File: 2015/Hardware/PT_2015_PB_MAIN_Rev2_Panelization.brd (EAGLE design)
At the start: 142.5 x 234.8 mm, 161 parts, among them Q1 Q_ACS711LC_SKETCH, Q11 Q_IRFS7437PbF, Q12 2N7002, Q14 Q_IRFS7437PbF, Q16 Q_IRFS7437PbF, Q18 Q_FDT86102LZ, Q20 Q_IRFS7437PbF, Q4 Q_ACS711LC, Q5 Q_ACS711LC, Q6 Q_IRFS7437PbF, Q7 Q_IRFS7437PbF, Q9 Q_IRFS7437PbF

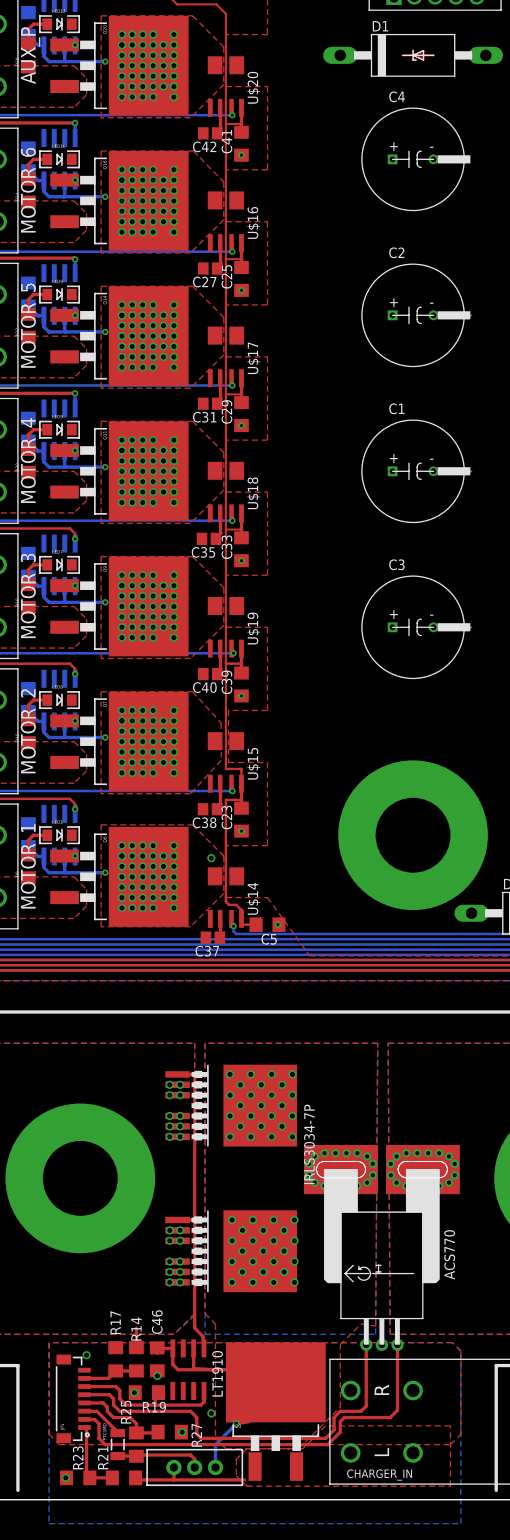
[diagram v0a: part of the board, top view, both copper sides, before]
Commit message: Cleaned up my idiotic TSTOP
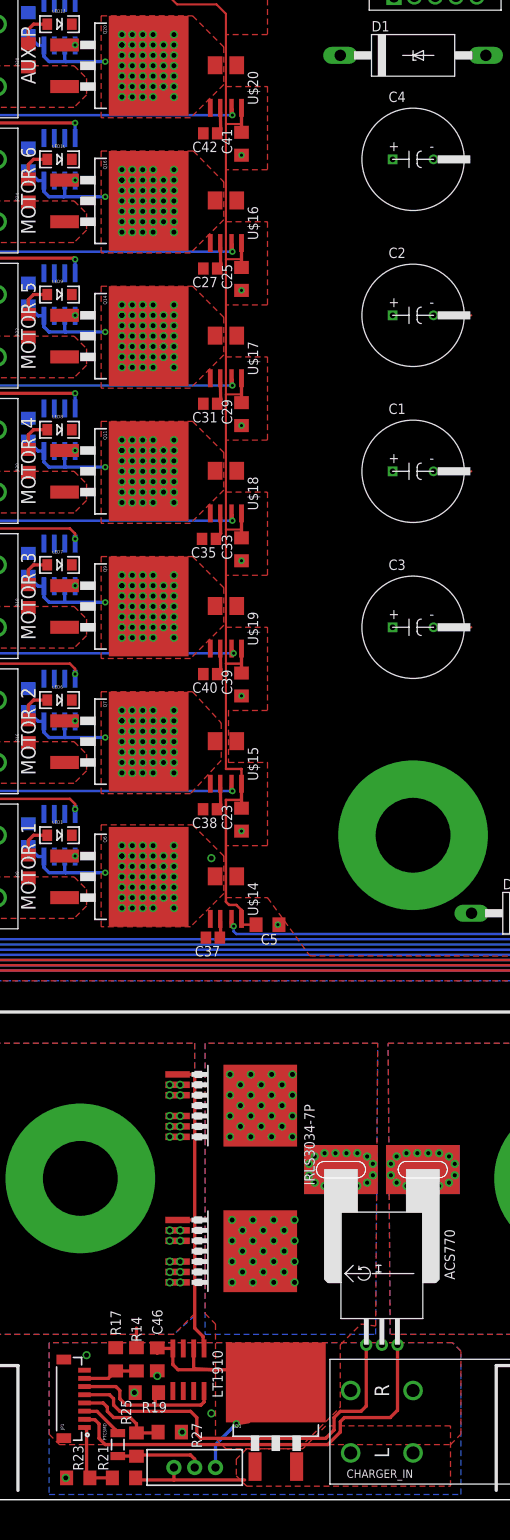
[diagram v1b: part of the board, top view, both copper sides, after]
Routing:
- net N$33: track 10.2 -> 0.00 mm
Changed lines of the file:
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@@
 <vertex x="5.08" y="2.54"/>
 </polygon>
-<dimension x1="137.795" y1="166.37" x2="137.795" y2="-67.945" x3="180.34" y3="49.2125" textsize="1.778" layer="21" unit="inch"/>
 <wire x1="1.27" y1="-8.89" x2="104.14" y2="-8.89" width="0.4064" layer="21"/>
 <wire x1="1.27" y1="-8.89" x2="1.27" y2="-52.07" width="0.4064" layer="21"/>
@@
 <wire x1="73.66" y1="-52.07" x2="104.14" y2="-52.07" width="0.4064" layer="21"/>
 <wire x1="104.14" y1="-52.07" x2="104.14" y2="-8.89" width="0.4064" layer="21"/>
+<dimension x1="137.795" y1="166.37" x2="137.541" y2="-68.453" x3="165.69279375" y3="48.928184375" textsize="3.81" layer="29" unit="inch" visible="yes"/>
 <polygon width="0.8128" layer="29">
-<vertex x="45.466" y="119.888"/>
-<vertex x="45.466" y="110.998"/>
-<vertex x="40.894" y="110.998"/>
-<vertex x="40.894" y="103.886"/>
-<vertex x="45.466" y="103.886"/>
-<vertex x="57.658" y="103.886"/>
-<vertex x="57.658" y="105.918"/>
-<vertex x="51.562" y="105.918"/>
-<vertex x="51.562" y="109.728"/>
-<vertex x="51.562" y="111.506"/>
-<vertex x="62.992" y="111.506"/>
-<vertex x="75.184" y="111.506"/>
-<vertex x="75.184" y="105.918"/>
-<vertex x="69.342" y="105.918"/>
-<vertex x="69.342" y="104.14"/>
-<vertex x="82.042" y="104.14"/>
-<vertex x="82.042" y="120.396"/>
-<vertex x="45.466" y="120.396"/>
+<vertex x="71.882" y="1.27"/>
+<vertex x="71.882" y="1.27"/>
+<vertex x="72.136" y="1.27"/>
 </polygon>
 <polygon width="0.8128" layer="29">
-<vertex x="57.658" y="104.902"/>
-<vertex x="69.342" y="104.902"/>
-<vertex x="69.342" y="104.14"/>
-<vertex x="57.658" y="104.14"/>
-<vertex x="57.658" y="103.886"/>
-</polygon>
-<polygon width="0.8128" layer="29">
-<vertex x="63.754" y="104.394"/>
-<vertex x="63.754" y="101.854"/>
-<vertex x="64.516" y="101.854" curve="-90"/>
-<vertex x="71.12" y="95.25" curve="-96.025575"/>
-<vertex x="63.5" y="88.392"/>
-<vertex x="63.5" y="83.058"/>
-<vertex x="64.516" y="83.058" curve="-90"/>
-<vertex x="71.374" y="76.2" curve="-97.62815"/>
-<vertex x="63.246" y="69.088"/>
-<vertex x="63.5" y="69.088"/>
-<vertex x="63.5" y="64.008"/>
-<vertex x="64.516" y="64.008" curve="-90"/>
-<vertex x="71.374" y="57.15" curve="-95.631113"/>
-<vertex x="63.246" y="49.784"/>
-<vertex x="63.246" y="44.958"/>
-<vertex x="64.77" y="44.958" curve="-90"/>
-<vertex x="71.628" y="38.1" curve="-90"/>
-<vertex x="64.516" y="30.988"/>
-<vertex x="63.246" y="30.988"/>
-<vertex x="63.246" y="6.35"/>
-<vertex x="81.026" y="6.35"/>
-<vertex x="81.026" y="23.622"/>
-<vertex x="79.248" y="23.622"/>
-<vertex x="79.248" y="26.67"/>
-<vertex x="81.026" y="26.67"/>
-<vertex x="81.026" y="53.594"/>
-<vertex x="80.01" y="53.594"/>
-<vertex x="80.01" y="104.14"/>
-<vertex x="73.914" y="104.14"/>
-<vertex x="73.914" y="104.394"/>
-</polygon>
-<polygon width="0.8128" layer="29">
-<vertex x="62.992" y="104.648"/>
-<vertex x="62.992" y="102.108"/>
-<vertex x="62.738" y="102.108" curve="90"/>
-<vertex x="56.642" y="96.012"/>
-<vertex x="56.642" y="94.742"/>
-<vertex x="56.642" y="94.488" curve="90"/>
-<vertex x="62.738" y="88.392" curve="-90"/>
-<vertex x="62.992" y="88.138"/>
-<vertex x="62.992" y="83.058"/>
-<vertex x="62.738" y="83.058" curve="90"/>
-<vertex x="56.642" y="76.962"/>
-<vertex x="56.642" y="75.692" curve="90"/>
-<vertex x="63.246" y="69.088"/>
-<vertex x="63.246" y="64.008"/>
-<vertex x="62.992" y="64.008" curve="90"/>
-<vertex x="56.642" y="57.658"/>
-<vertex x="56.642" y="56.642" curve="90"/>
-<vertex x="62.738" y="50.546"/>
-<vertex x="62.738" y="45.212" curve="90"/>
-<vertex x="56.642" y="39.116"/>
-<vertex x="56.642" y="37.592" curve="90"/>
-<vertex x="62.992" y="31.242"/>
-<vertex x="63.246" y="31.242"/>
-<vertex x="63.246" y="-1.778"/>
-<vertex x="60.198" y="-1.778"/>
-<vertex x="51.562" y="-1.778"/>
-<vertex x="49.784" y="0"/>
-<vertex x="48.514" y="1.27"/>
-<vertex x="48.514" y="2.54"/>
-<vertex x="48.514" y="3.302"/>
-<vertex x="47.498" y="3.302"/>
-<vertex x="47.498" y="5.334"/>
+<vertex x="45.974" y="120.65"/>
+<vertex x="45.974" y="110.236"/>
+<vertex x="41.402" y="110.236"/>
+<vertex x="41.402" y="104.394"/>
+<vertex x="45.974" y="104.394"/>
+<vertex x="45.974" y="93.726"/>
+<vertex x="41.402" y="93.726"/>
+<vertex x="41.402" y="87.884"/>
+<vertex x="45.974" y="87.884"/>
+<vertex x="45.974" y="77.216"/>
+<vertex x="41.402" y="77.216"/>
+<vertex x="41.402" y="71.374"/>
+<vertex x="45.974" y="71.374"/>
+<vertex x="45.974" y="60.706"/>
+<vertex x="41.402" y="60.706"/>
+<vertex x="41.402" y="54.864"/>
+<vertex x="45.974" y="54.864"/>
+<vertex x="45.974" y="44.196"/>
+<vertex x="41.402" y="44.196"/>
+<vertex x="41.402" y="38.354"/>
+<vertex x="45.974" y="38.354"/>
+<vertex x="45.974" y="27.686"/>
+<vertex x="41.402" y="27.686"/>
+<vertex x="41.402" y="21.844"/>
+<vertex x="45.974" y="21.844"/>
+<vertex x="45.974" y="11.176"/>
+<vertex x="41.402" y="11.176"/>
 <vertex x="41.402" y="5.334"/>
-<vertex x="41.402" y="11.176"/>
-<vertex x="45.72" y="11.176"/>
-<vertex x="45.974" y="11.176"/>
-<vertex x="45.974" y="21.844"/>
-<vertex x="41.402" y="21.844"/>
-<vertex x="41.402" y="27.686"/>
-<vertex x="45.974" y="27.686"/>
-<vertex x="45.974" y="38.354"/>
-<vertex x="45.72" y="38.354"/>
-<vertex x="41.402" y="38.354"/>
-<vertex x="41.402" y="44.196"/>
-<vertex x="45.974" y="44.196"/>
-<vertex x="45.974" y="54.864"/>
-<vertex x="41.402" y="54.864"/>
-<vertex x="41.402" y="60.706"/>
-<vertex x="46.228" y="60.706"/>
-<vertex x="45.974" y="60.706"/>
-<vertex x="45.974" y="71.374"/>
-<vertex x="41.402" y="71.374"/>
-<vertex x="41.402" y="77.216"/>
-<vertex x="45.974" y="77.216"/>
-<vertex x="45.974" y="87.884"/>
-<vertex x="41.402" y="87.884"/>
-<vertex x="41.402" y="93.726"/>
-<vertex x="45.974" y="93.726"/>
-<vertex x="45.974" y="104.648"/>
-</polygon>
-<polygon width="0.8128" layer="29">
-<vertex x="63.5" y="-1.778"/>
-<vertex x="67.818" y="-1.778"/>
-<vertex x="67.818" y="2.794"/>
-<vertex x="67.818" y="5.08"/>
-<vertex x="71.12" y="5.08"/>
-<vertex x="73.914" y="5.08"/>
-<vertex x="73.914" y="6.35"/>
-<vertex x="81.026" y="6.35"/>
-<vertex x="81.026" y="8.128"/>
-<vertex x="79.248" y="8.128"/>
-<vertex x="63.5" y="8.128"/>
-</polygon>
-<polygon width="0.8128" layer="29">
-<vertex x="67.818" y="1.524"/>
-<vertex x="67.818" y="1.27"/>
-<vertex x="72.136" y="1.27"/>
-<vertex x="72.136" y="0"/>
-<vertex x="81.026" y="0"/>
+<vertex x="45.974" y="5.334"/>
+<vertex x="49.53" y="5.334"/>
+<vertex x="49.53" y="0.508"/>
+<vertex x="53.086" y="0.508"/>
+<vertex x="53.086" y="-1.778"/>
+<vertex x="60.96" y="-1.778"/>
 <vertex x="81.026" y="-1.778"/>
-<vertex x="67.818" y="-1.778"/>
-<vertex x="67.818" y="1.27"/>
+<vertex x="81.026" y="12.954"/>
+<vertex x="79.248" y="12.954"/>
+<vertex x="79.248" y="34.29"/>
+<vertex x="81.026" y="34.29"/>
+<vertex x="81.026" y="36.83"/>
+<vertex x="81.026" y="47.752"/>
+<vertex x="79.502" y="47.752"/>
+<vertex x="79.502" y="55.118"/>
+<vertex x="79.502" y="71.628"/>
+<vertex x="79.756" y="71.628"/>
+<vertex x="79.756" y="119.126"/>
+<vertex x="79.756" y="119.888"/>
+<vertex x="77.47" y="119.888"/>
+<vertex x="57.404" y="119.888"/>
+<vertex x="57.404" y="113.03"/>
+<vertex x="75.438" y="113.03"/>
+<vertex x="75.438" y="104.14"/>
+<vertex x="57.404" y="104.14"/>
+<vertex x="57.404" y="113.03"/>
+<vertex x="57.404" y="98.044"/>
+<vertex x="72.136" y="98.044"/>
+<vertex x="72.136" y="92.71"/>
+<vertex x="57.404" y="92.71"/>
+<vertex x="57.404" y="98.044"/>
+<vertex x="57.404" y="73.406"/>
+<vertex x="72.39" y="73.406"/>
+<vertex x="72.39" y="80.01"/>
+<vertex x="57.404" y="80.01"/>
+<vertex x="57.404" y="54.61"/>
+<vertex x="72.136" y="54.61"/>
+<vertex x="72.136" y="60.198"/>
+<vertex x="57.404" y="60.198"/>
+<vertex x="57.404" y="35.56"/>
+<vertex x="72.898" y="35.56"/>
+<vertex x="72.898" y="42.672"/>
+<vertex x="57.404" y="42.672"/>
+<vertex x="57.404" y="120.396"/>
+<vertex x="45.974" y="120.396"/>
 </polygon>
 </plain>
@@
 <vertex x="68.326" y="-49.276"/>
 <vertex x="19.05" y="-49.276"/>
-<vertex x="19.05" y="-71.374"/>
-<vertex x="69.342" y="-71.374"/>
+<vertex x="19.05" y="-67.818"/>
+<vertex x="69.342" y="-67.818"/>
 <vertex x="69.342" y="-50.292"/>
 </polygon>
@@
 <wire x1="97.79" y1="46.863" x2="97.79" y2="44.2625" width="0.3048" layer="1"/>
 </signal>
-<signal name="N$33">
-<wire x1="62.23" y1="107.95" x2="63.5" y2="107.95" width="0.254" layer="1"/>
-<wire x1="63.5" y1="107.95" x2="63.627" y2="107.95" width="0.254" layer="1"/>
-<wire x1="63.627" y1="107.95" x2="64.77" y2="107.95" width="0.254" layer="1"/>
-<wire x1="66.04" y1="107.95" x2="64.77" y2="107.95" width="0.254" layer="1"/>
-<wire x1="64.77" y1="107.95" x2="64.77" y2="108.458" width="0.254" layer="1"/>
-<wire x1="64.77" y1="108.458" x2="63.627" y2="107.95" width="0.254" layer="1"/>
-<wire x1="63.627" y1="107.95" x2="64.77" y2="107.442" width="0.254" layer="1"/>
-<wire x1="64.77" y1="107.442" x2="64.77" y2="107.95" width="0.254" layer="1"/>
-<wire x1="64.77" y1="108.458" x2="63.5" y2="107.95" width="0.254" layer="1"/>
-<wire x1="63.5" y1="107.95" x2="63.5" y2="108.585" width="0.254" layer="1"/>
-<wire x1="63.5" y1="107.95" x2="63.5" y2="107.442" width="0.254" layer="1"/>
-<wire x1="63.5" y1="107.442" x2="63.881" y2="107.442" width="0.254" layer="1"/>
-</signal>
 <signal name="N$34">
